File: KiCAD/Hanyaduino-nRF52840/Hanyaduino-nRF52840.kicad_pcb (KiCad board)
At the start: 2 copper layers, 35.1 x 17.8 mm, 29 parts, among them J1 Conn_01x03_Female, J4 USB_B_Micro, Q1 DMG3415U, U1 MCP73831-2-OT, U2 BL654(nRF52840), U3 AP2113(3.3V)

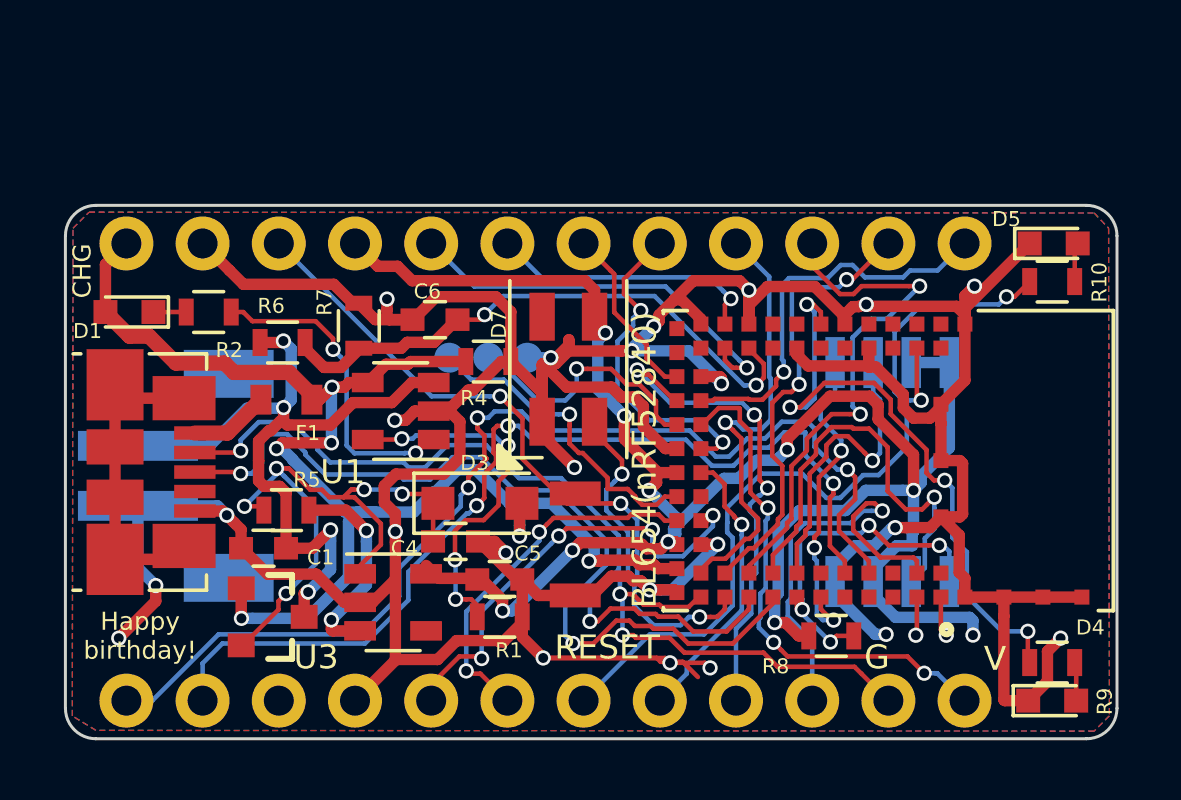
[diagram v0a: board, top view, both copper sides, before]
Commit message: Hanyaduino-nRF52840 v1.0
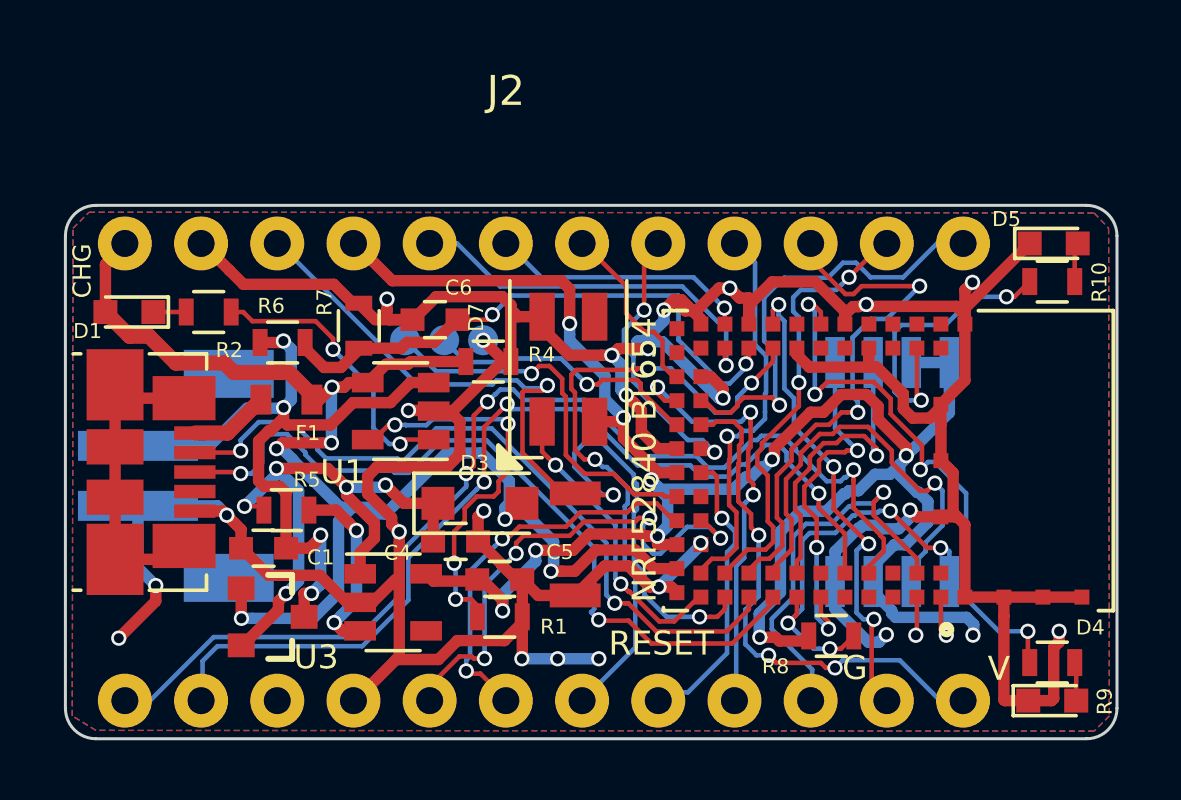
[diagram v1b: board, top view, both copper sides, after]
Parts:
- removed e: Arduino_pro_micro_conn, library:Arduino_pro_micro_conn
- added J2: Arduino_pro_micro_conn, library:Arduino_pro_micro_conn, F.Cu at (126.9, 114.3)
- added REF**: OSHW-Logo2_7.3x6mm_SilkScreen, KiCAD footprints:OSHW-Logo2_7.3x6mm_SilkScreen, B.Cu at (124.6, 119.5)
- D7: value SK6812 -> SK6812MINI
- U2: value BL654(nRF52840) -> NRF52840 BL654
- moved J1 1.58 mm to (124.9, 112.4)
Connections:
- D7 pad 1: VCC -> Net-(D7-Pad1)
- D7 pad 2: Net-(D7-Pad2) -> GND
- D7 pad 3: GND -> D8/NeoPixel
- D7 pad 4: D8/NeoPixel -> VCC
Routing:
- net D18/A4: track 0.00 -> 21.6 mm, vias 0 -> 3
- net D4/LED2: track 28.7 -> 10.00 mm
- net D19/A5: track 0.00 -> 16.9 mm, vias 0 -> 4
- net GND: track 164.4 -> 149.7 mm, vias 23 -> 24
- net D8/NeoPixel: track 21.6 -> 10.0 mm, vias 3 -> 2
- net RESET: track 23.4 -> 30.1 mm
- net D+: track 29.0 -> 26.2 mm
- net D12/RX: track 10.5 -> 12.8 mm
- net D-: track 26.7 -> 24.6 mm
- net D6: track 16.7 -> 14.6 mm
- net D28/CS(QSPI): track 11.8 -> 13.5 mm
- net D22/SDA(I2C): track 15.2 -> 16.9 mm
- net D3/LED1: track 20.5 -> 18.9 mm
- net D10: track 13.2 -> 14.8 mm
- net D26/SCK(SPI): track 14.7 -> 13.3 mm
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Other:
- board text added: "+"
- board text added: "-"
- board text added: "Hanyaduino nRF52840 Rev 1.0 Dec 16, 2018"
- board text removed: "Hanyaduino nRF52840 Rev 0.81 Dec 11, 2018"
- board text removed: "Happy birthday!"
